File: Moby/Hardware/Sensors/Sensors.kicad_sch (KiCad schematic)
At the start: 4 parts, among them U6 MS5607-02BA

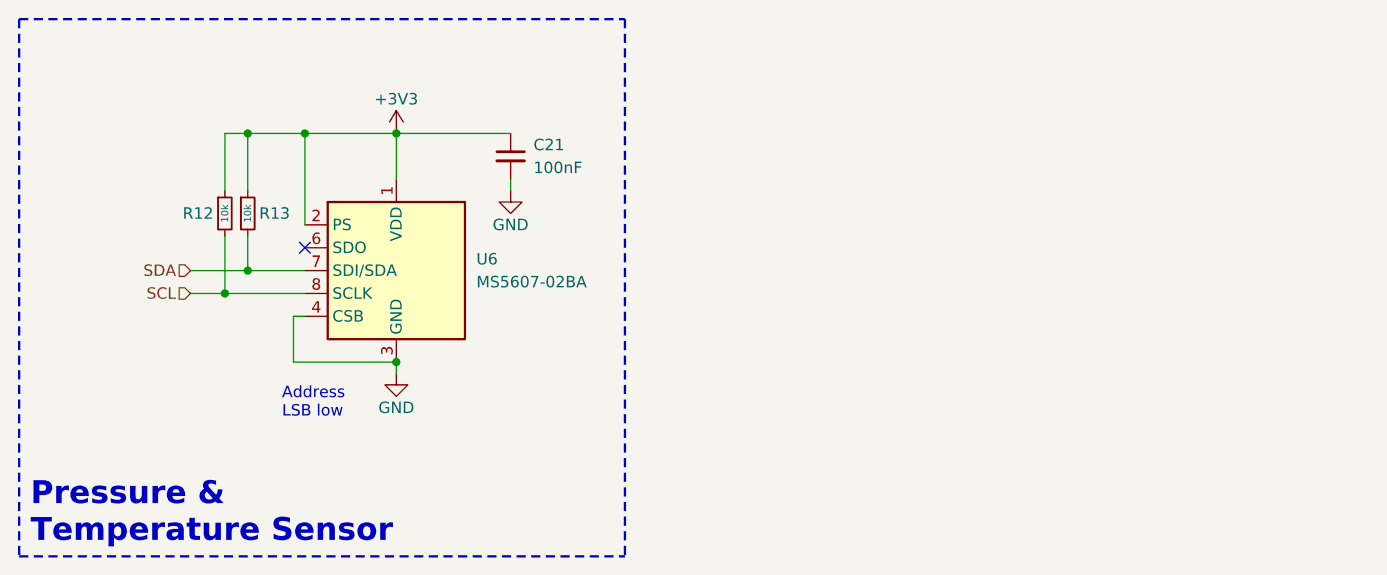
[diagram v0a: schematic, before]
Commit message: I think I added the IMU mostly
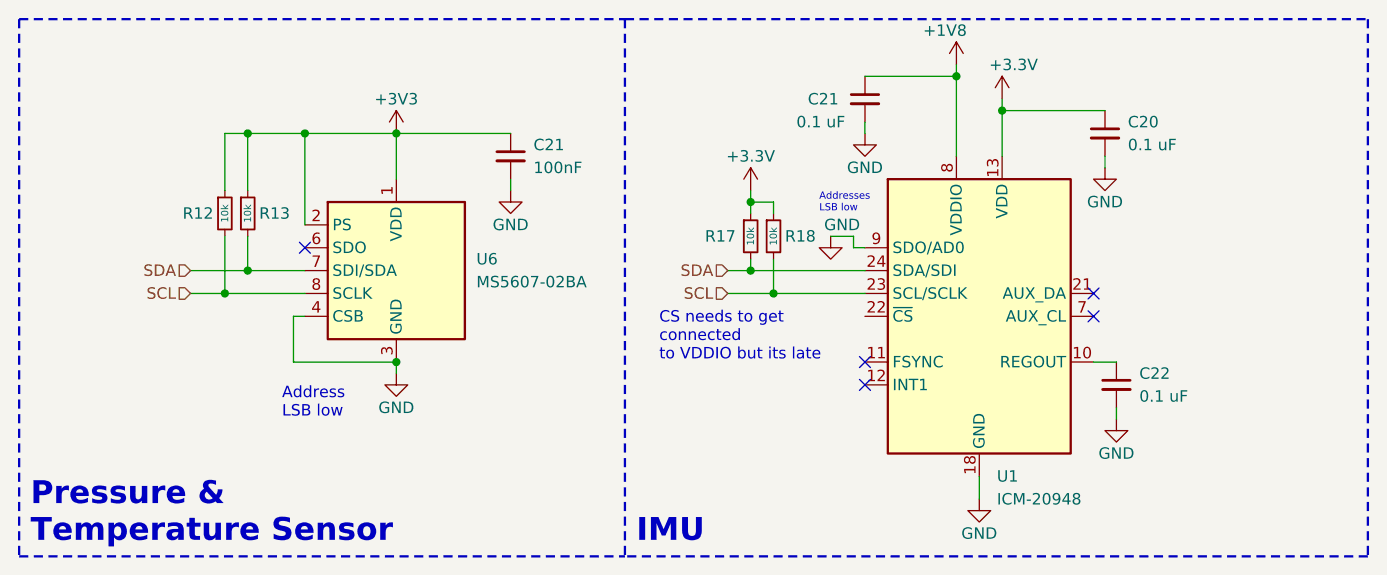
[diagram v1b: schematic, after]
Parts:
- added C20, C21, C22: 0.1 uF, symbol Device:C_Small
- added R17, R18: 10k, symbol Device:R_Small
- added U1: ICM-20948, Sensor_Motion:InvenSense_QFN-24_3x3mm_P0.4mm, symbol Sensor_Motion:ICM-20948
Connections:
- net GND: now also C20.2, C21.2, C22.2, U1.18 (GND), U1.20 (GND), U1.9 (SDO/AD0)
- net SCL: now also R18.2, U1.23 (SCL/SCLK)
- net SDA: now also R17.2, U1.24 (SDA/SDI)
- new net: C22.1, U1.10 (REGOUT)
- new net +1V8: C21.1, U1.8 (VDDIO)
- new net +3.3V: C20.1, R17.1, R18.1, U1.13 (VDD)
- no-connect marks 1 -> 5
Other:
- note added: "Addresses LSB low"
- note added: "CS needs to get connected to VDDIO but its late"
- note added: "IMU"
